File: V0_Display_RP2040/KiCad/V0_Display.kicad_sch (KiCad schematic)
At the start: 46 parts, among them J1 USB4145-03-0230-C_REVA2, J2 I2C Header 1, J3 SWD, J7 USB_Header, J8 Conn_01x02, SW1 RESET, SW5 BOOTSEL, SW6 Killswitch, SW7 Rotary_Encoder_Switch, U1 AP2127K-3.3, U2 USBLC6-2P6, U3 74LVC1G17, U4 W25Q16JVUXIQ_TR, U5 RP2040, Y1 12Mhz

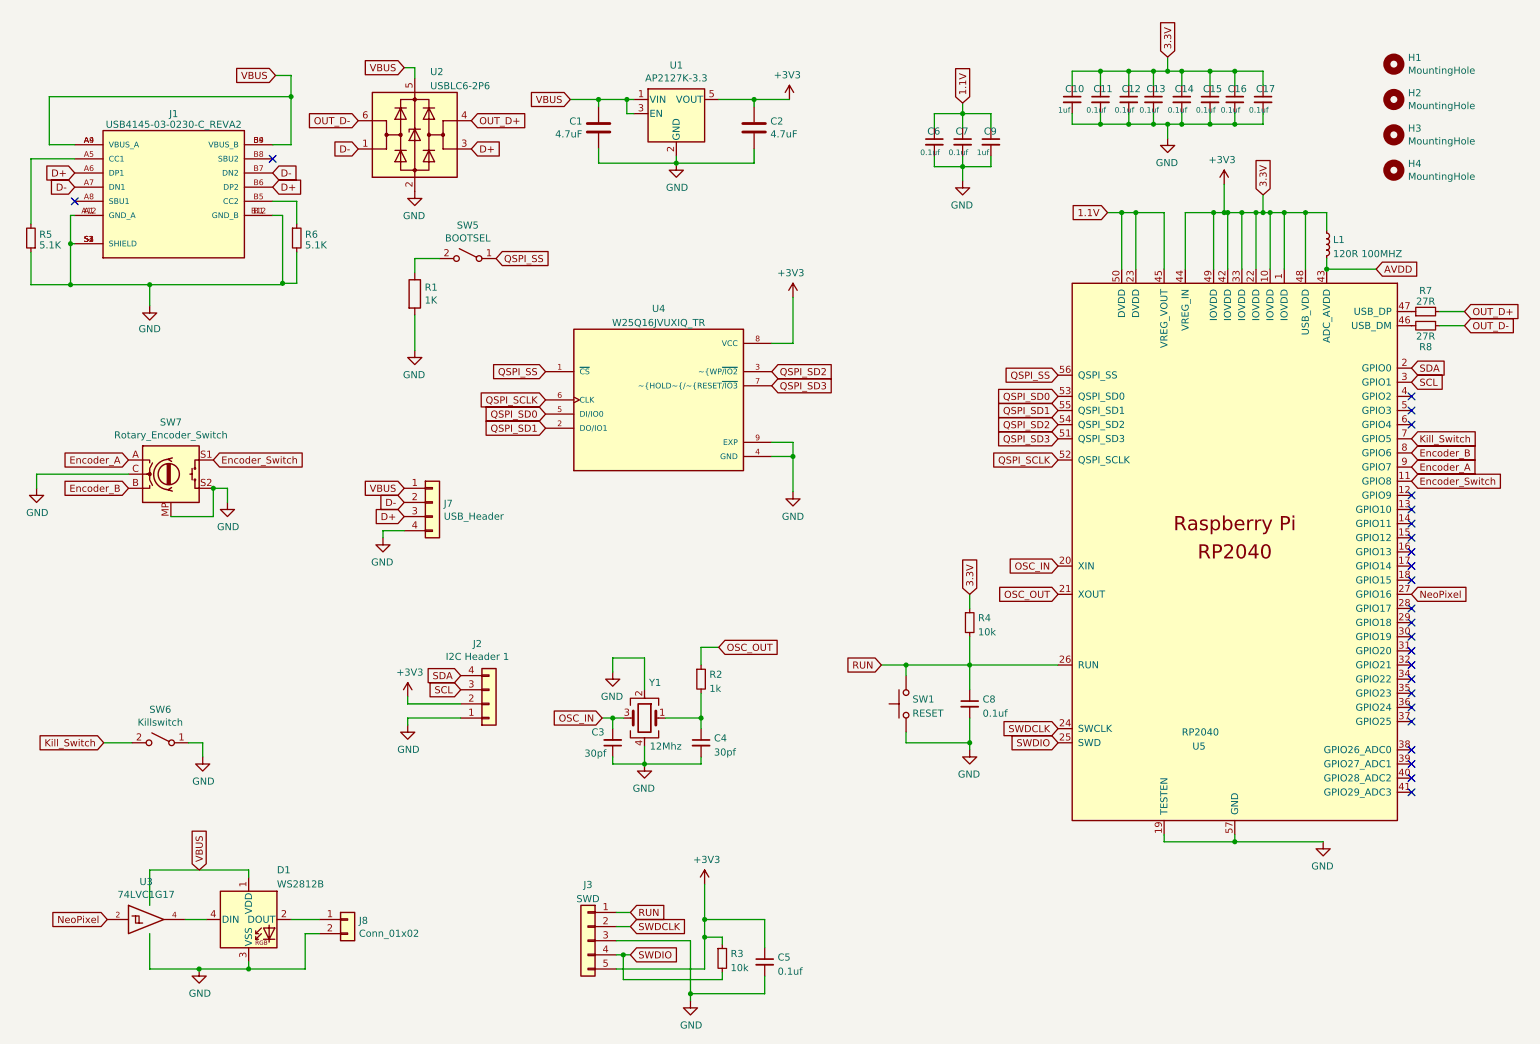
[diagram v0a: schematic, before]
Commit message: Usability updates to hardware
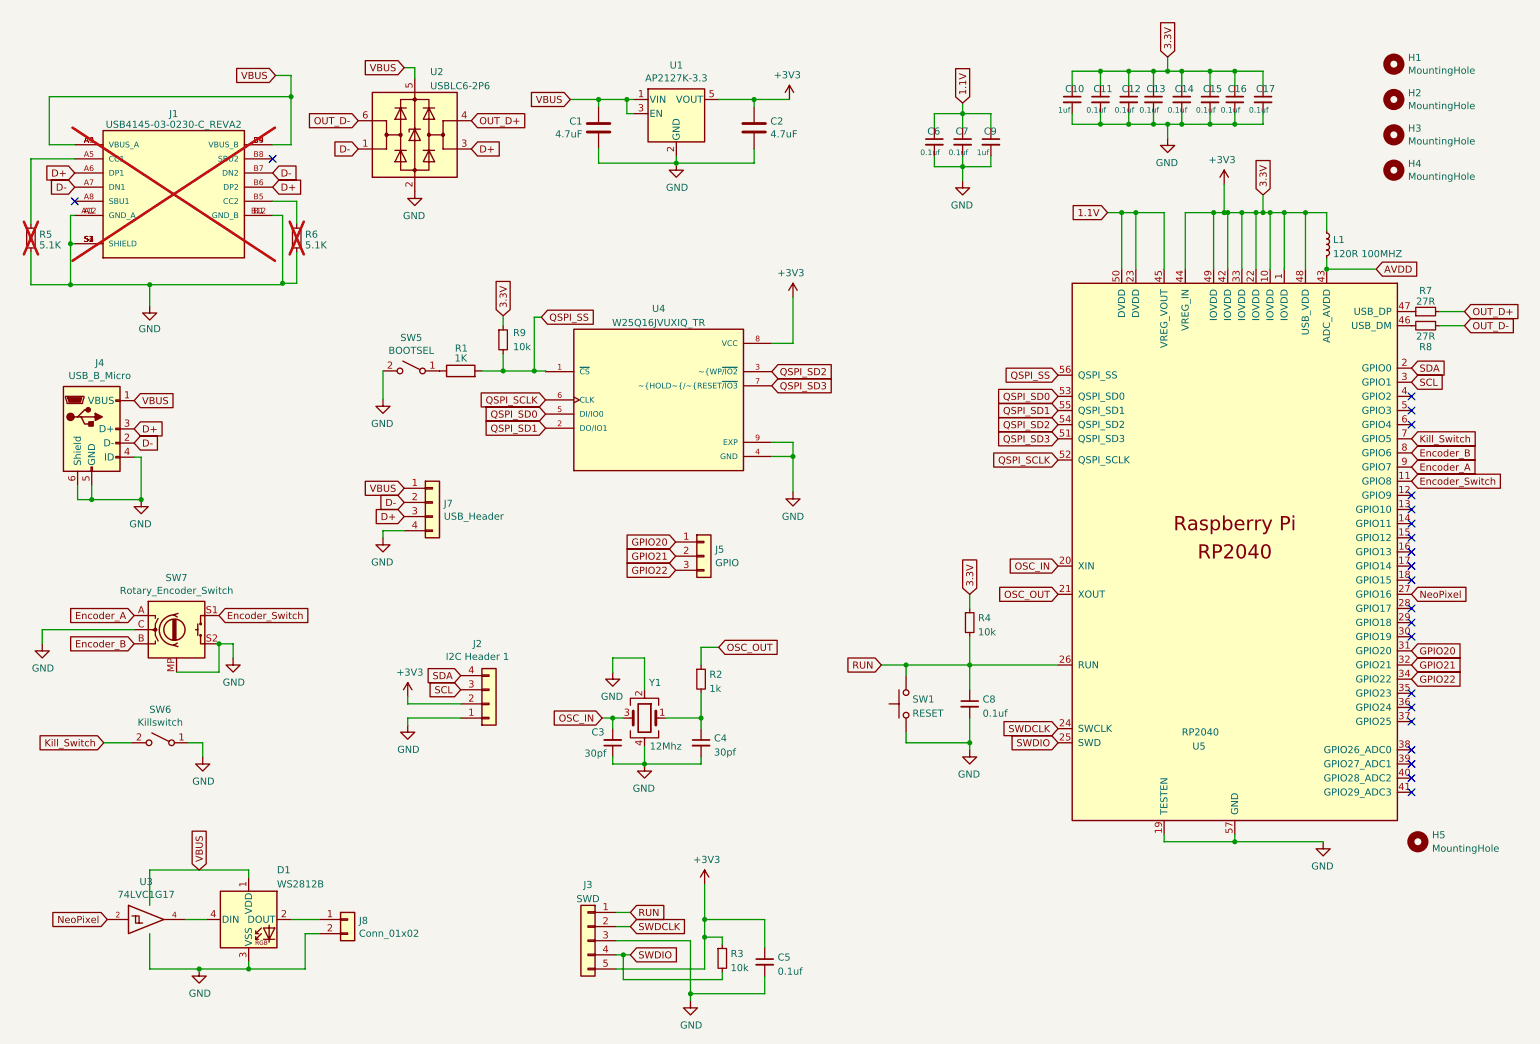
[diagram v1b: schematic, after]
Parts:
- added H5: MountingHole, Library:VoronLogo_6pt5mm_silkScreen, symbol Library:MountingHole
- added J4: USB_B_Micro, Library:MolexVertical&Horizontal_MicroB, symbol Library:USB_B_Micro
- added J5: GPIO, Connector_PinHeader_2.54mm:PinHeader_1x03_P2.54mm_Vertical, symbol Library:Conn_01x03
- added R9: 10k, Voron0 2040 display:R_0603_1608Metric, symbol Library:R_Small
- C1, C2: symbol Voron0 2040 display:C -> Library:C
- C10, C11, C12, C13, C14, C15, C16, C17, C3, C4, C5, C6, C7, C8, C9: symbol Voron0 2040 display:C_Small -> Library:C_Small
- D1: symbol Voron0 2040 display:WS2812B -> Library:WS2812B
- H1, H2, H3, H4: symbol Voron0 2040 display:MountingHole -> Library:MountingHole
- J1: symbol USB4145-03-0230-C_REVA2:USB4145-03-0230-C_REVA2 -> Library:USB4145-03-0230-C_REVA2; now not fitted
- J2: footprint Voron0 2040 display:1pt3in_OLED -> Library:1pt3in_OLED; symbol Voron0 2040 display:Conn_01x04 -> Library:Conn_01x04
- J3: symbol Voron0 2040 display:Conn_01x05 -> Library:Conn_01x05
- J7: symbol Voron0 2040 display:Conn_01x04 -> Library:Conn_01x04
- J8: symbol Voron0 2040 display:Conn_01x02 -> Library:Conn_01x02
- L1: symbol Voron0 2040 display:L_Small -> Library:L_Small
- R1: symbol Voron0 2040 display:R -> Library:R
- R2, R3, R4: symbol Voron0 2040 display:R_Small -> Library:R_Small
- R5, R6: symbol Voron0 2040 display:R_Small -> Library:R_Small; now not fitted
- R7, R8: symbol Device:R_Small -> Library:R_Small
- SW1: symbol Voron0 2040 display:SW_Push -> Library:SW_Push
- SW5, SW6: symbol Voron0 2040 display:SW_SPST -> Library:SW_SPST
- SW7: symbol Voron0 2040 display:Rotary_Encoder_Switch -> Library:Rotary_Encoder_Switch
- U1: symbol Voron0 2040 display:AP2127K-3.3 -> Library:AP2127K-3.3
- U2: symbol Voron0 2040 display:USBLC6-2P6 -> Library:USBLC6-2P6
- U3: symbol Voron0 2040 display:74LVC1G17 -> Library:74LVC1G17
- U4: symbol Voron0 2040 display:W25Q16JVUXIQ_TR -> Library:W25Q16JVUXIQ_TR
- U5: symbol Voron0 2040 display:RP2040 -> Library:RP2040
- Y1: symbol Voron0 2040 display:Crystal_GND24 -> Library:Crystal_GND24
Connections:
- net +3V3: now also R9.1
- net D+: now also J4.3 (D+)
- net D-: now also J4.2 (D-)
- net GND: now also SW5.2 (B), J4.4 (ID), J4.5 (GND), J4.6 (Shield); no longer R1.2
- net QSPI_SS: now also R1.2, R9.2; no longer SW5.1 (A)
- net VCC: now also J4.1 (VBUS)
- net at R1.1: now also SW5.1 (A); no longer SW5.2 (B)
- net GPIO20: now reaches U5.31 (GPIO20)
- net GPIO20: now also J5.1 (Pin_1)
- net GPIO21: now reaches U5.32 (GPIO21)
- net GPIO21: now also J5.2 (Pin_2)
- net GPIO22: now reaches U5.34 (GPIO22)
- net GPIO22: now also J5.3 (Pin_3)
- no-connect marks 25 -> 22
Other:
- moved on the sheet: R1, SW5, SW7

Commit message: Clean up
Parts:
- C1, C2: footprint Voron0 2040 display:C_0603_1608Metric -> Library:C_0603_1608Metric; LCSC C326580 -> C19666
- C10, C9: footprint Voron0 2040 display:C_0402_1005Metric -> Library:C_0402_1005Metric; LCSC C106254 -> C52923
- C11, C12, C13, C14, C15, C16, C17, C5, C6, C7, C8: footprint Voron0 2040 display:C_0402_1005Metric -> Library:C_0402_1005Metric; LCSC C129131 -> C1525
- C3, C4: footprint Voron0 2040 display:C_0402_1005Metric -> Library:C_0402_1005Metric
- D1: footprint Voron0 2040 display:LED_WS2812B_PLCC4_5.0x5.0mm_P3.2mm -> Library:LED_WS2812B_PLCC4_5.0x5.0mm_P3.2mm; LCSC C114586 -> C2761795
- H1, H2, H3, H4: footprint Voron0 2040 display:MountingHole_3.2mm_M3 -> Library:MountingHole_3.2mm_M3
- J1: footprint USB4145-03-0230-C_REVA2:GCT_USB4145-03-0230-C_REVA2 -> Library:GCT_USB4145-03-0230-C_REVA2; Availability In Stock -> (none); Check_prices https://www.snapeda.com/parts/USB4145-03-0230-C/Global+Conn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 -> (none); MANUFACTURER GCT -> (none); MAXIMUM_PACKAGE_HEIGHT 7.66mm -> (none); MF Global Connector Technology -> (none); MP USB4145-03-0230-C -> (none); MPN (none) -> USB4145-03-0230-C; PARTREV A2 -> (none); Package None -> (none); Price None -> (none); SNAPEDA_PN USB4145-03-0230-C -> (none); STANDARD Manufacturer Recommendations -> (none); SnapEDA_Link https://www.snapeda.com/parts/USB4145-03-0230-C/Global+Conn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 -> (none)
- J3: footprint Voron0 2040 display:PinHeader_1x05_P2.54mm_Vertical -> Library:PinHeader_1x05_P2.54mm_Vertical
- J7: footprint Voron0 2040 display:PinHeader_1x04_P2.54mm_Vertical -> Library:PinHeader_1x04_P2.54mm_Vertical
- J8: footprint Voron0 2040 display:PinHeader_1x02_P2.54mm_Vertical -> Library:PinHeader_1x02_P2.54mm_Vertical
- L1: footprint Voron0 2040 display:L_0402_1005Metric -> Library:L_0402_1005Metric
- R1: footprint Voron0 2040 display:R_0603_1608Metric -> Library:R_0603_1608Metric; LCSC C4295595 -> C21190
- R2: footprint Voron0 2040 display:R_0402_1005Metric -> Library:R_0603_1608Metric; LCSC C852624 -> C21190
- R3, R4, R9: footprint Voron0 2040 display:R_0603_1608Metric -> Library:R_0603_1608Metric; LCSC C2139679 -> C25804
- R5, R6: footprint Voron0 2040 display:R_0402_1005Metric -> Library:R_0603_1608Metric; LCSC C105873 -> C23186
- R7, R8: footprint Voron0 2040 display:R_0402_1005Metric -> Library:R_0402_1005Metric
- SW7: footprint Voron0 2040 display:EN11_Encoder -> Library:EN11_Encoder
- U1: footprint Voron0 2040 display:SOT-23-5 -> Library:SOT-23-5
- U2: footprint Voron0 2040 display:SOT-666 -> Library:SOT-666
- U3: footprint Voron0 2040 display:SOT-753 -> Library:SOT-753
- U4: footprint Voron0 2040 display:IC_W25Q16JVUXIQ_TR -> Library:IC_W25Q16JVUXIQ_TR
- U5: footprint Voron0 2040 display:RP2040-QFN-56 -> Library:RP2040-QFN-56
- Y1: footprint Voron0 2040 display:Crystal_SMD_3225-4Pin_3.2x2.5mm -> Library:Crystal_SMD_3225-4Pin_3.2x2.5mm

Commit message: Fixed up gerbers
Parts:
- H5, J1, R5, R6: now left out of the parts list
- J4: LCSC (none) -> C136000
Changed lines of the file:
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@@
+      (effects (font (size 1.27 1.27)) hide)
+    )
+    (property "LCSC" "C136000" (at 27.686 85.852 0)
       (effects (font (size 1.27 1.27)) hide)
     )
@@
   )
   (symbol (lib_id "Library:MountingHole") (at 265.938 160.02 0) (unit 1)
-    (in_bom yes) (on_board yes) (dnp no) (fields_autoplaced)
+    (in_bom no) (on_board yes) (dnp no) (fields_autoplaced)
     (property "Reference" "H5" (at 268.478 158.8079 0)
       (effects (font (size 1.27 1.27)) (justify left))
@@
     )
     (property "Datasheet" "~" (at 265.938 160.02 0)
+      (effects (font (size 1.27 1.27)) hide)
+    )
+    (property "Sim.Enable" "0" (at 265.938 160.02 0)
       (effects (font (size 1.27 1.27)) hide)
     )
@@
   )
   (symbol (lib_id "Library:USB4145-03-0230-C_REVA2") (at 42.418 42.418 0) (unit 1)
-    (in_bom yes) (on_board no) (dnp yes) (fields_autoplaced)
+    (in_bom no) (on_board no) (dnp yes) (fields_autoplaced)
     (property "Reference" "J1" (at 42.418 29.2481 0)
       (effects (font (size 1.27 1.27)))
@@
   )
   (symbol (lib_id "Library:R_Small") (at 64.516 51.562 0) (unit 1)
-    (in_bom yes) (on_board no) (dnp yes) (fields_autoplaced)
+    (in_bom no) (on_board no) (dnp yes) (fields_autoplaced)
     (property "Reference" "R6" (at 66.0146 50.9183 0)
       (effects (font (size 1.27 1.27)) (justify left))
@@
   )
   (symbol (lib_id "Library:R_Small") (at 16.764 51.562 180) (unit 1)
-    (in_bom yes) (on_board no) (dnp yes) (fields_autoplaced)
+    (in_bom no) (on_board no) (dnp yes) (fields_autoplaced)
     (property "Reference" "R5" (at 18.2626 50.9183 0)
       (effects (font (size 1.27 1.27)) (justify right))
